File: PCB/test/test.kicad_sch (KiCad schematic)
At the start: 54 parts, among them CN5 UFL, SW2 MLL1200S_TE, U1 STM32WBxx_QFN48, U2 USBLC6-2SC6, U3 LD3985M33R, X1 NX2016_32MHz, X2 NX2012_32K768Hz

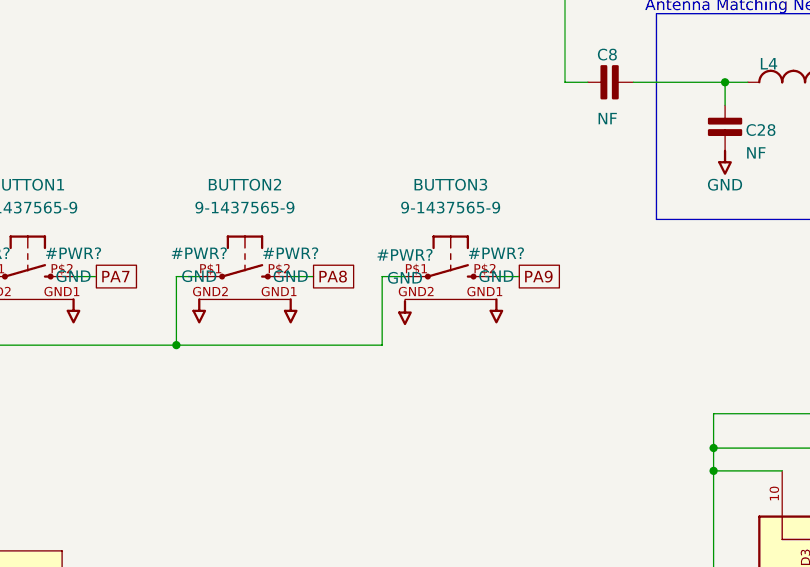
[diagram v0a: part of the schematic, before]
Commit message: small error fixes
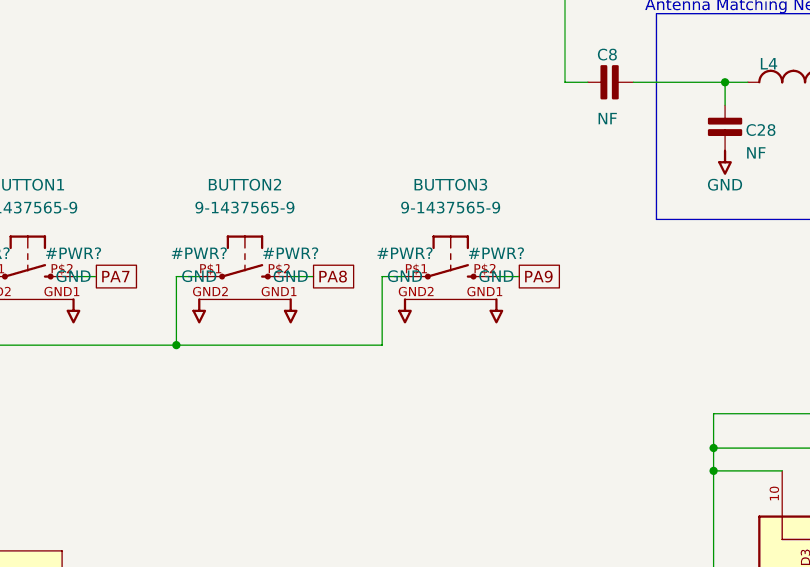
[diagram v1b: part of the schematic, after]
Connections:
- net GND: now also BUTTON3.GND2
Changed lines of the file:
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@@
     (pin "")
   )
-  (symbol (lib_id "test-altium-import:GND") (at 190.5 144.9656 0) (unit 1)
+  (symbol (lib_id "test-altium-import:GND") (at 190.5 144.78 0) (unit 1)
     (in_bom yes) (on_board yes) (fields_autoplaced)
-    (property "Reference" "#PWR?" (id 0) (at 190.5 139.8856 0))
-    (property "Value" "GND" (id 1) (at 190.5 142.4256 0))
-    (property "Footprint" "" (id 2) (at 190.5 144.9656 0)
+    (property "Reference" "#PWR?" (id 0) (at 190.5 139.7 0))
+    (property "Value" "GND" (id 1) (at 190.5 142.24 0))
+    (property "Footprint" "" (id 2) (at 190.5 144.78 0)
       (effects (font (size 1.27 1.27)) hide)
     )
-    (property "Datasheet" "" (id 3) (at 190.5 144.9656 0)
+    (property "Datasheet" "" (id 3) (at 190.5 144.78 0)
       (effects (font (size 1.27 1.27)) hide)
     )
